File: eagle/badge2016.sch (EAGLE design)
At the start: 123 parts, among them IC1 25AA080SN, IC2 FT231XQ, J1 USB-MICRO, Q2 BC857ALT1SMD, Q2_24MHZ NX5032G, X1 PASSER-07, X10 PAD-1.27X1.27, X11 PAD-1.27X1.27, X12 PAD-1.27X1.27, X13 PAD-1.27X1.27, X14 PAD-1.27X1.27, X15 PAD-1.27X1.27, X16 PAD-1.27X1.27, X17 PAD-1.27X1.27, X18 PAD-1.27X1.27, X19 PAD-1.27X1.27, X2 PASSER-07, X20 PAD-1.27X1.27, X21 PAD-0.5, X3 PASSER-07, X4 PAD-0.5, X5 PAD-0.5, X6 PAD-0.5, X7 PAD-0.5, X8 PAD-1.27X1.27, X9 PAD-1.27X1.27

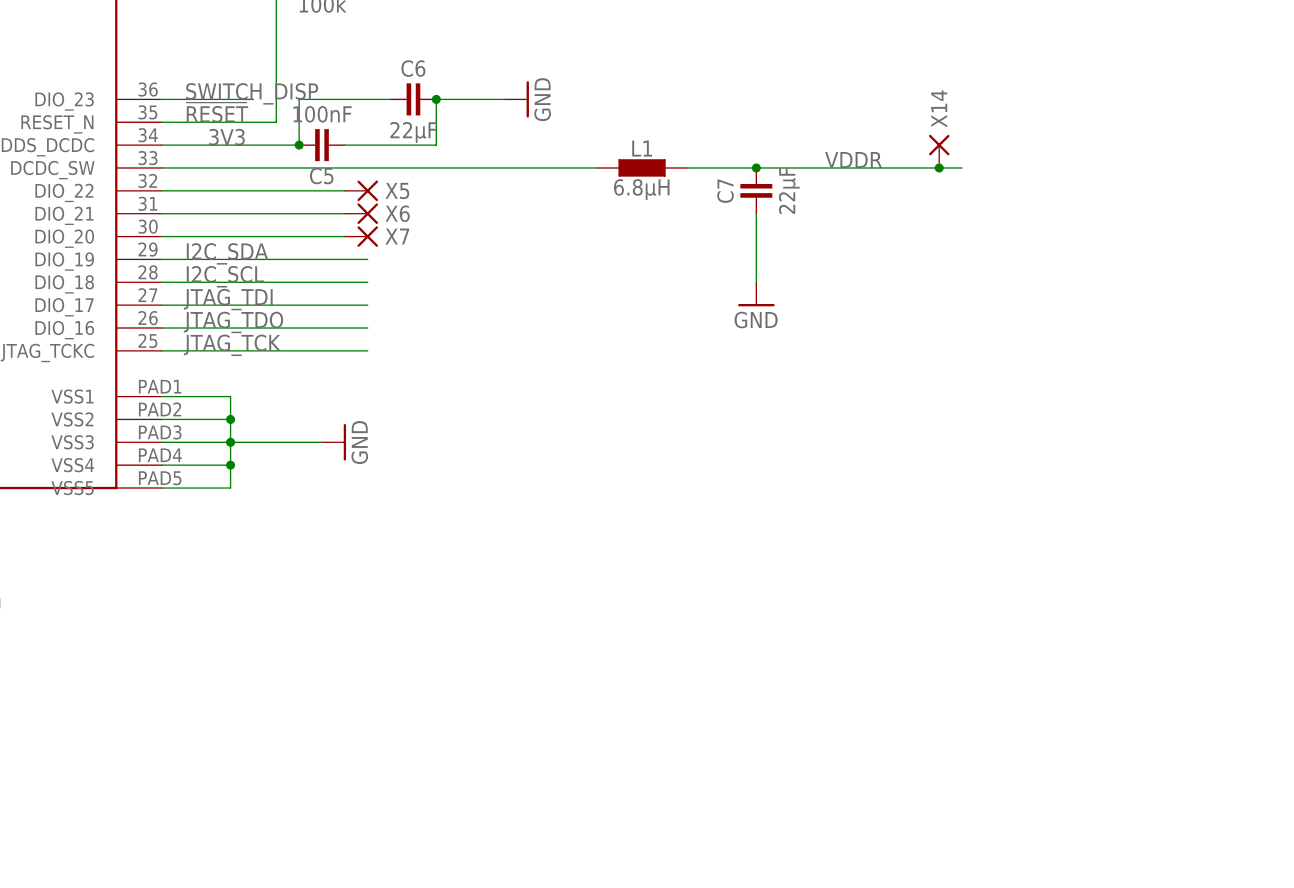
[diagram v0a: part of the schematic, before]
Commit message: newest pcb state
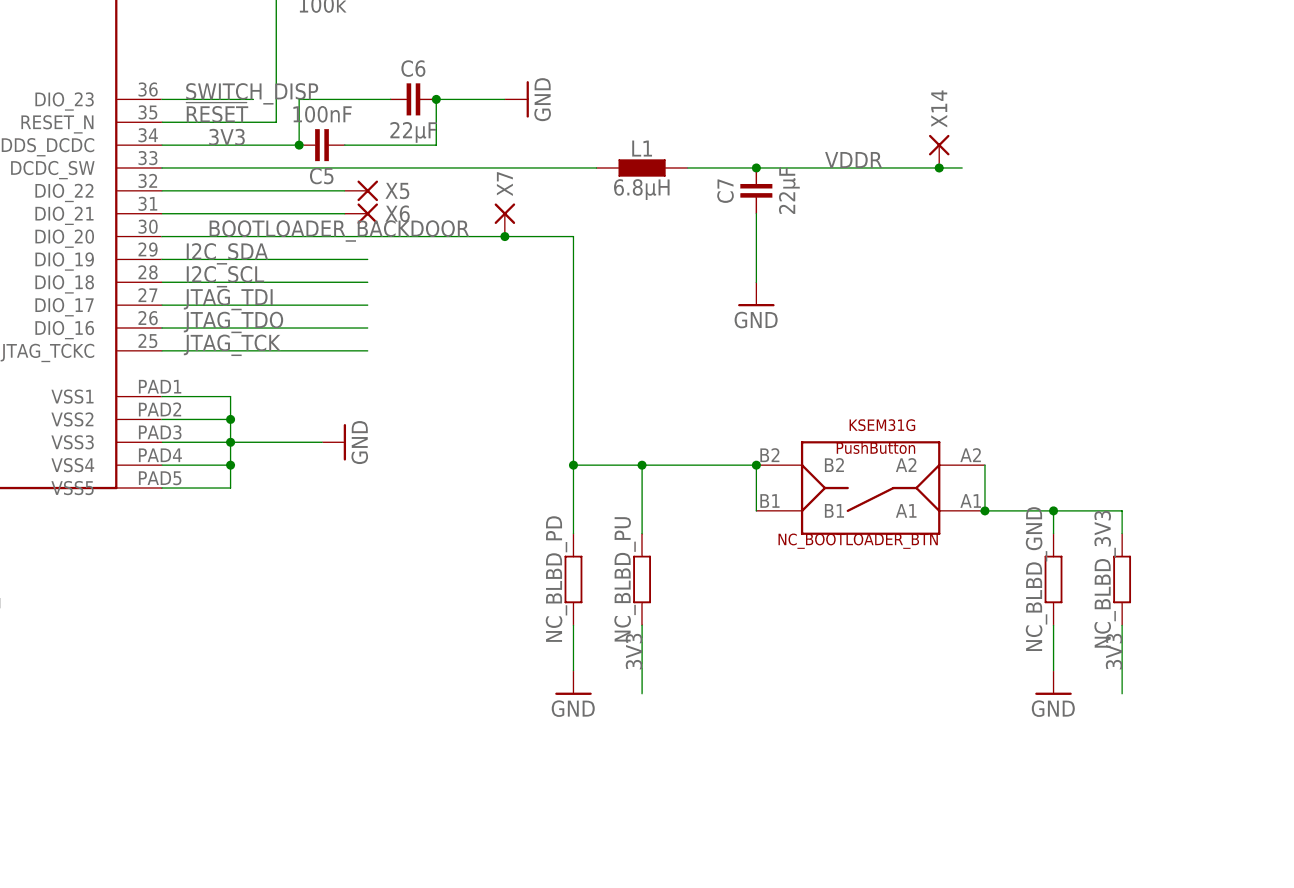
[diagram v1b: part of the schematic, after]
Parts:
- added NC_BLBD_3V3, NC_BLBD_GND, NC_BLBD_PD, NC_BLBD_PU: (no value), we-rcl:RESISTOR-0402
- added NC_BOOTLOADER_BTN: KSEM31G, ERNW_parts:KSEM31G
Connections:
- removed net N$38: U$1.DIO_20, X7.P
- new net BOOTLOADER_BACKDOOR: NC_BLBD_PD.2, NC_BLBD_PU.2, NC_BOOTLOADER_BTN.B1, NC_BOOTLOADER_BTN.B2, U$1.DIO_20, X7.P
- new net N$55: NC_BLBD_3V3.2, NC_BLBD_GND.2, NC_BOOTLOADER_BTN.A1, NC_BOOTLOADER_BTN.A2
- net 3V3: now also NC_BLBD_3V3.1, NC_BLBD_PU.1
- net GND: now also NC_BLBD_GND.1, NC_BLBD_PD.1
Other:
- moved on the sheet: X7
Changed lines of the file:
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@@
 <part name="R15" library="we-rcl" deviceset="RESISTOR" device="-0402" value="0R3"/>
 <part name="GND53" library="supply1" deviceset="GND" device=""/>
+<part name="NC_BOOTLOADER_BTN" library="ERNW_parts" deviceset="KSEM31G" device=""/>
+<part name="NC_BLBD_PD" library="we-rcl" deviceset="RESISTOR" device="-0402"/>
+<part name="NC_BLBD_PU" library="we-rcl" deviceset="RESISTOR" device="-0402"/>
+<part name="NC_BLBD_GND" library="we-rcl" deviceset="RESISTOR" device="-0402"/>
+<part name="NC_BLBD_3V3" library="we-rcl" deviceset="RESISTOR" device="-0402"/>
+<part name="GND59" library="supply1" deviceset="GND" device=""/>
+<part name="GND60" library="supply1" deviceset="GND" device=""/>
 </parts>
 <sheets>
@@
 <instance part="X5" gate="X" x="114.3" y="45.72" rot="R180"/>
 <instance part="X6" gate="X" x="114.3" y="43.18" rot="R180"/>
-<instance part="X7" gate="X" x="114.3" y="40.64" rot="R180"/>
+<instance part="X7" gate="X" x="129.54" y="43.18" rot="R270"/>
 <instance part="X8" gate="X" x="-142.24" y="-269.24" rot="R90"/>
 <instance part="X9" gate="X" x="-142.24" y="-261.62" rot="R270"/>
@@
 <instance part="R15" gate="R" x="45.72" y="-264.16"/>
 <instance part="GND53" gate="1" x="55.88" y="-264.16" rot="R90"/>
+<instance part="NC_BOOTLOADER_BTN" gate="G$1" x="170.18" y="12.7" rot="R180"/>
+<instance part="NC_BLBD_PD" gate="R" x="137.16" y="2.54" rot="R90"/>
+<instance part="NC_BLBD_PU" gate="R" x="144.78" y="2.54" rot="R90"/>
+<instance part="NC_BLBD_GND" gate="R" x="190.5" y="2.54" rot="R90"/>
+<instance part="NC_BLBD_3V3" gate="R" x="198.12" y="2.54" rot="R90"/>
+<instance part="GND59" gate="1" x="137.16" y="-10.16"/>
+<instance part="GND60" gate="1" x="190.5" y="-10.16"/>
 </instances>
 <busses>
@@
 <wire x1="53.34" y1="-264.16" x2="50.8" y2="-264.16" width="0.1524" layer="91"/>
 </segment>
+<segment>
+<pinref part="NC_BLBD_PD" gate="R" pin="1"/>
+<pinref part="GND59" gate="1" pin="GND"/>
+<wire x1="137.16" y1="-2.54" x2="137.16" y2="-7.62" width="0.1524" layer="91"/>
+</segment>
+<segment>
+<pinref part="NC_BLBD_GND" gate="R" pin="1"/>
+<pinref part="GND60" gate="1" pin="GND"/>
+<wire x1="190.5" y1="-2.54" x2="190.5" y2="-7.62" width="0.1524" layer="91"/>
+</segment>
 </net>
 <net name="3V3" class="0">
@@
 <wire x1="218.44" y1="-187.96" x2="218.44" y2="-185.42" width="0.1524" layer="91"/>
 <junction x="218.44" y="-185.42"/>
+</segment>
+<segment>
+<pinref part="NC_BLBD_PU" gate="R" pin="1"/>
+<wire x1="144.78" y1="-2.54" x2="144.78" y2="-10.16" width="0.1524" layer="91"/>
+<label x="144.78" y="-7.62" size="1.778" layer="95" rot="R90"/>
+</segment>
+<segment>
+<pinref part="NC_BLBD_3V3" gate="R" pin="1"/>
+<wire x1="198.12" y1="-2.54" x2="198.12" y2="-10.16" width="0.1524" layer="91"/>
+<label x="198.12" y="-7.62" size="1.778" layer="95" rot="R90"/>
 </segment>
 </net>
@@
 </segment>
 </net>
-<net name="N$38" class="0">
+<net name="BOOTLOADER_BACKDOOR" class="0">
 <segment>
 <pinref part="U$1" gate="G$1" pin="DIO_20"/>
 <pinref part="X7" gate="X" pin="P"/>
-<wire x1="91.44" y1="40.64" x2="111.76" y2="40.64" width="0.1524" layer="91"/>
+<wire x1="91.44" y1="40.64" x2="129.54" y2="40.64" width="0.1524" layer="91"/>
+<wire x1="129.54" y1="40.64" x2="137.16" y2="40.64" width="0.1524" layer="91"/>
+<wire x1="137.16" y1="40.64" x2="137.16" y2="15.24" width="0.1524" layer="91"/>
+<junction x="129.54" y="40.64"/>
+<pinref part="NC_BOOTLOADER_BTN" gate="G$1" pin="B2"/>
+<wire x1="137.16" y1="15.24" x2="144.78" y2="15.24" width="0.1524" layer="91"/>
+<pinref part="NC_BLBD_PD" gate="R" pin="2"/>
+<wire x1="144.78" y1="15.24" x2="157.48" y2="15.24" width="0.1524" layer="91"/>
+<wire x1="137.16" y1="15.24" x2="137.16" y2="7.62" width="0.1524" layer="91"/>
+<junction x="137.16" y="15.24"/>
+<pinref part="NC_BLBD_PU" gate="R" pin="2"/>
+<wire x1="144.78" y1="15.24" x2="144.78" y2="7.62" width="0.1524" layer="91"/>
+<junction x="144.78" y="15.24"/>
+<pinref part="NC_BOOTLOADER_BTN" gate="G$1" pin="B1"/>
+<wire x1="157.48" y1="15.24" x2="157.48" y2="10.16" width="0.1524" layer="91"/>
+<junction x="157.48" y="15.24"/>
+<label x="96.52" y="40.64" size="1.778" layer="95"/>
 </segment>
 </net>
@@
 </segment>
 </net>
+<net name="N$55" class="0">
+<segment>
+<pinref part="NC_BOOTLOADER_BTN" gate="G$1" pin="A1"/>
+<pinref part="NC_BLBD_GND" gate="R" pin="2"/>
+<wire x1="182.88" y1="10.16" x2="190.5" y2="10.16" width="0.1524" layer="91"/>
+<wire x1="190.5" y1="10.16" x2="190.5" y2="7.62" width="0.1524" layer="91"/>
+<pinref part="NC_BLBD_3V3" gate="R" pin="2"/>
+<wire x1="190.5" y1="10.16" x2="198.12" y2="10.16" width="0.1524" layer="91"/>
+<wire x1="198.12" y1="10.16" x2="198.12" y2="7.62" width="0.1524" layer="91"/>
+<junction x="190.5" y="10.16"/>
+<pinref part="NC_BOOTLOADER_BTN" gate="G$1" pin="A2"/>
+<wire x1="182.88" y1="15.24" x2="182.88" y2="10.16" width="0.1524" layer="91"/>
+<junction x="182.88" y="10.16"/>
+</segment>
+</net>
